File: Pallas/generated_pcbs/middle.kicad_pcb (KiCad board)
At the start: 2 copper layers, 467.5 x 140 mm, 260 parts, among them J1 OLED, J2 RGB_LED, Q1 IRLML6344TRPbF, SW00 SW_PUSH, SW01 SW_PUSH, SW010 SW_PUSH, SW011 SW_PUSH, SW012 SW_PUSH, SW013 SW_PUSH, SW014 SW_PUSH, SW02 SW_PUSH, SW03 SW_PUSH, SW04 SW_PUSH, SW05 SW_PUSH, SW06 SW_PUSH, SW07 SW_PUSH, SW08 SW_PUSH, SW09 SW_PUSH, SW10 SW_PUSH, SW11 SW_PUSH, SW110 SW_PUSH, SW111 SW_PUSH, SW112 SW_PUSH, SW113 SW_PUSH, SW114 SW_PUSH, SW12 SW_PUSH, SW13 SW_PUSH, SW14 SW_PUSH, SW15 SW_PUSH, SW16 SW_PUSH, SW17 SW_PUSH, SW18 SW_PUSH, SW19 SW_PUSH, SW20 SW_PUSH, SW21 SW_PUSH, SW210 SW_PUSH, SW211 SW_PUSH, SW212 SW_PUSH, SW213 SW_PUSH, SW214 SW_PUSH, SW22 SW_PUSH, SW23 SW_PUSH, SW24 SW_PUSH, SW25 SW_PUSH, SW26 SW_PUSH, SW27 SW_PUSH, SW28 SW_PUSH, SW29 SW_PUSH, SW30 SW_PUSH, SW31 SW_PUSH, SW310 SW_PUSH, SW311 SW_PUSH, SW312 SW_PUSH, SW313 SW_PUSH, SW314 SW_PUSH, SW32 SW_PUSH, SW33 SW_PUSH, SW34 SW_PUSH, SW35 SW_PUSH, SW36 SW_PUSH, SW37 SW_PUSH, SW38 SW_PUSH, SW39 SW_PUSH, SW40 SW_PUSH, SW41 SW_PUSH, SW410 SW_PUSH, SW411 SW_PUSH, SW412 SW_PUSH, SW413 SW_PUSH, SW414 SW_PUSH, SW42 SW_PUSH, SW43 SW_PUSH, SW44 SW_PUSH, SW45 SW_PUSH, SW46 SW_PUSH, SW47 SW_PUSH, SW48 SW_PUSH, SW49 SW_PUSH, U1 Elite-C

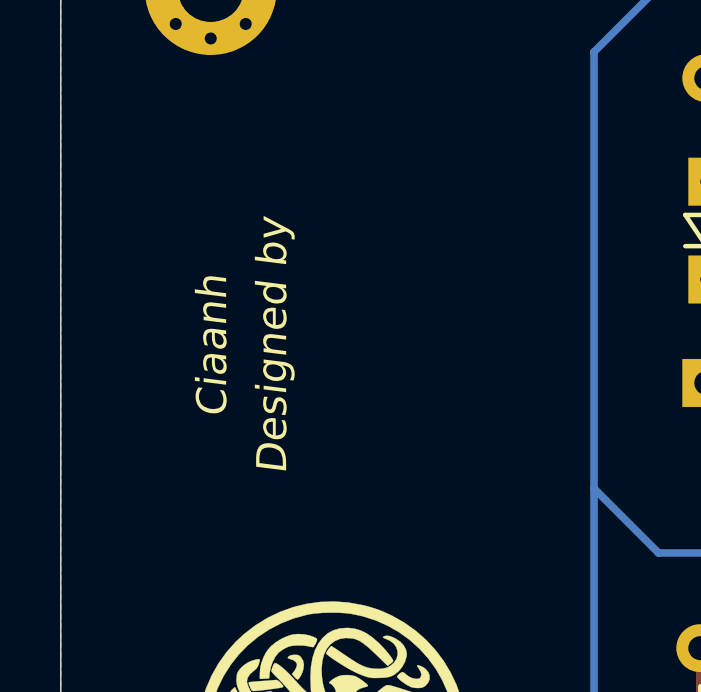
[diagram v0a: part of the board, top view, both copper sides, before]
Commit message: Fix issue with label design by
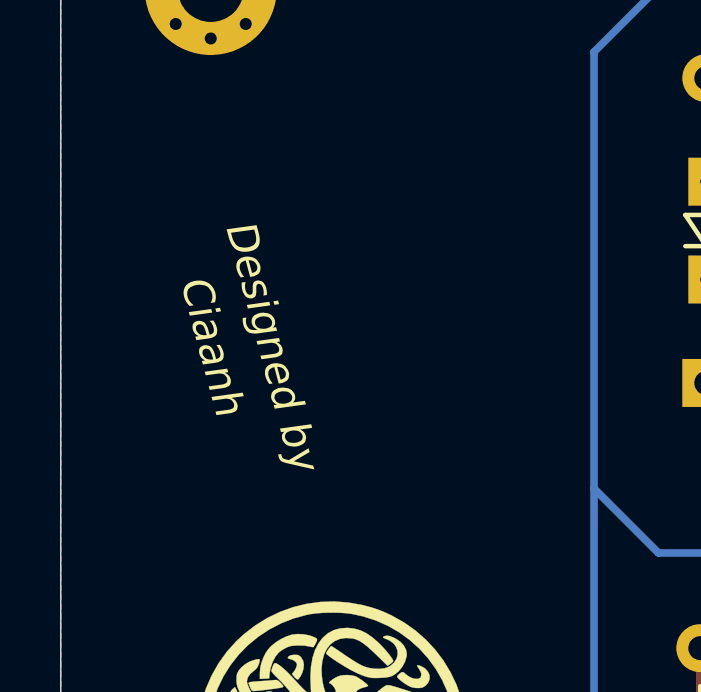
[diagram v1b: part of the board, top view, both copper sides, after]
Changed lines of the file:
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@@
-(kicad_pcb (version 20171130) (host pcbnew "(5.1.6)-1")
+(kicad_pcb (version 20171130) (host pcbnew 5.1.6-c6e7f7d~86~ubuntu20.04.1)
   (general
     (thickness 1.6)
@@
       (drillshape 0)
       (scaleselection 1)
-      (outputdirectory "gerber/middle/"))
+      (outputdirectory "pallas/"))
   )
   (net 0 "")
@@
       (xy -2.511352 -3.707233) (xy -2.125299 -3.941597) (xy -1.71799 -4.135869) (xy -1.29263 -4.288478)
       (xy -0.852427 -4.397857) (xy -0.400584 -4.462436) (xy 0.059691 -4.480646) (xy 0.525194 -4.450919)) (layer F.SilkS) (width 0.01))
-    (fp_text user Ciaanh (at -13 4 270) (layer B.SilkS)
+    (fp_text user Ciaanh (at -13 4 285) (layer B.SilkS)
       (effects (font (size 1 1) (thickness 0.15) italic) (justify mirror))
     )
-    (fp_text user "Designed by" (at -13 2 270) (layer B.SilkS)
+    (fp_text user "Designed by" (at -13 2 285) (layer B.SilkS)
       (effects (font (size 1 1) (thickness 0.15) italic) (justify mirror))
     )
-    (fp_text user Ciaanh (at -13 4 90) (layer F.SilkS)
+    (fp_text user Ciaanh (at -13 4 105) (layer F.SilkS)
       (effects (font (size 1 1) (thickness 0.15) italic))
     )
-    (fp_text user "Designed by" (at -13 2 90) (layer F.SilkS)
+    (fp_text user "Designed by" (at -13 2 105) (layer F.SilkS)
       (effects (font (size 1 1) (thickness 0.15) italic))
     )
